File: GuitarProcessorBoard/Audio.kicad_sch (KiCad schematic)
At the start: 44 parts, among them U201 TLV320AIC3204, U202 TL074

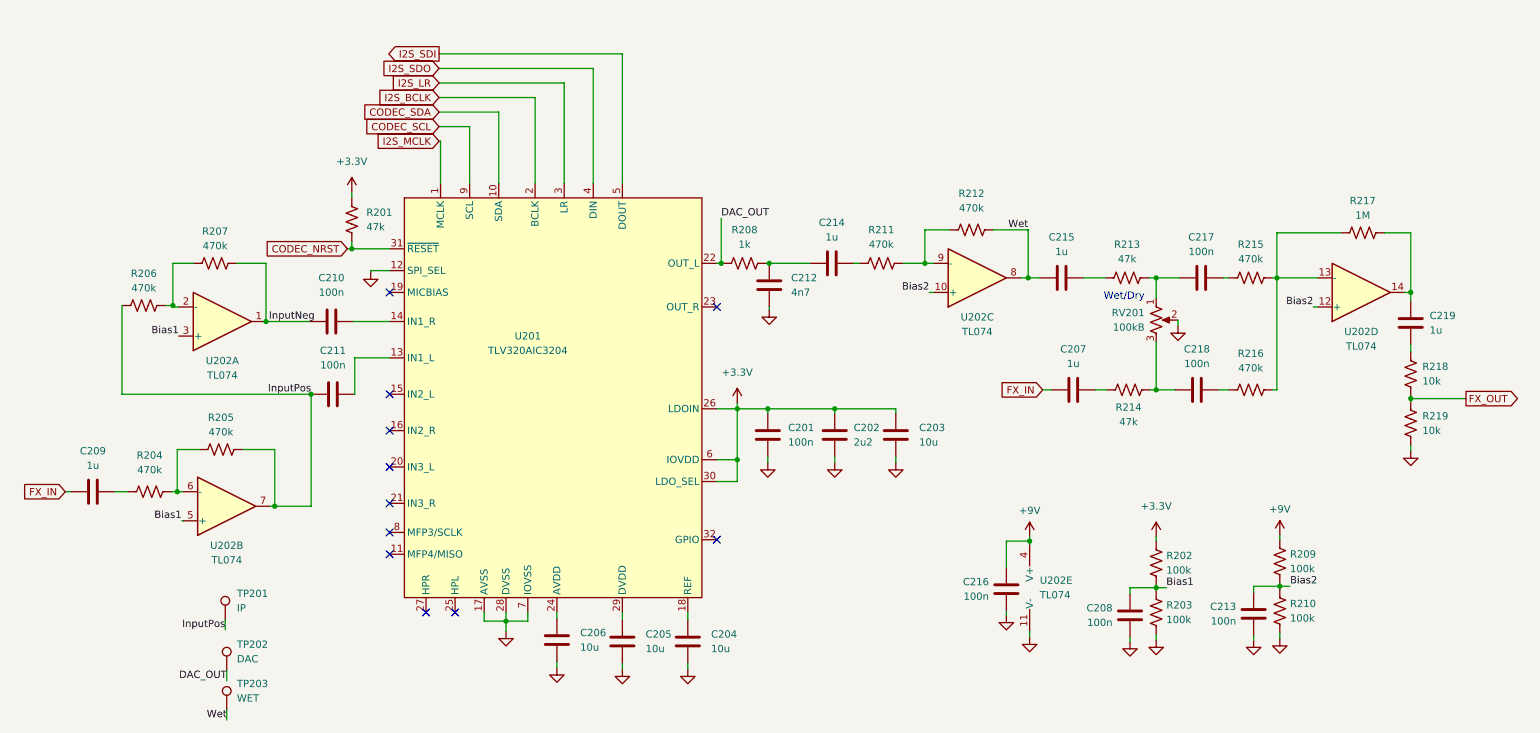
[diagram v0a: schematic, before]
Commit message: starting layout
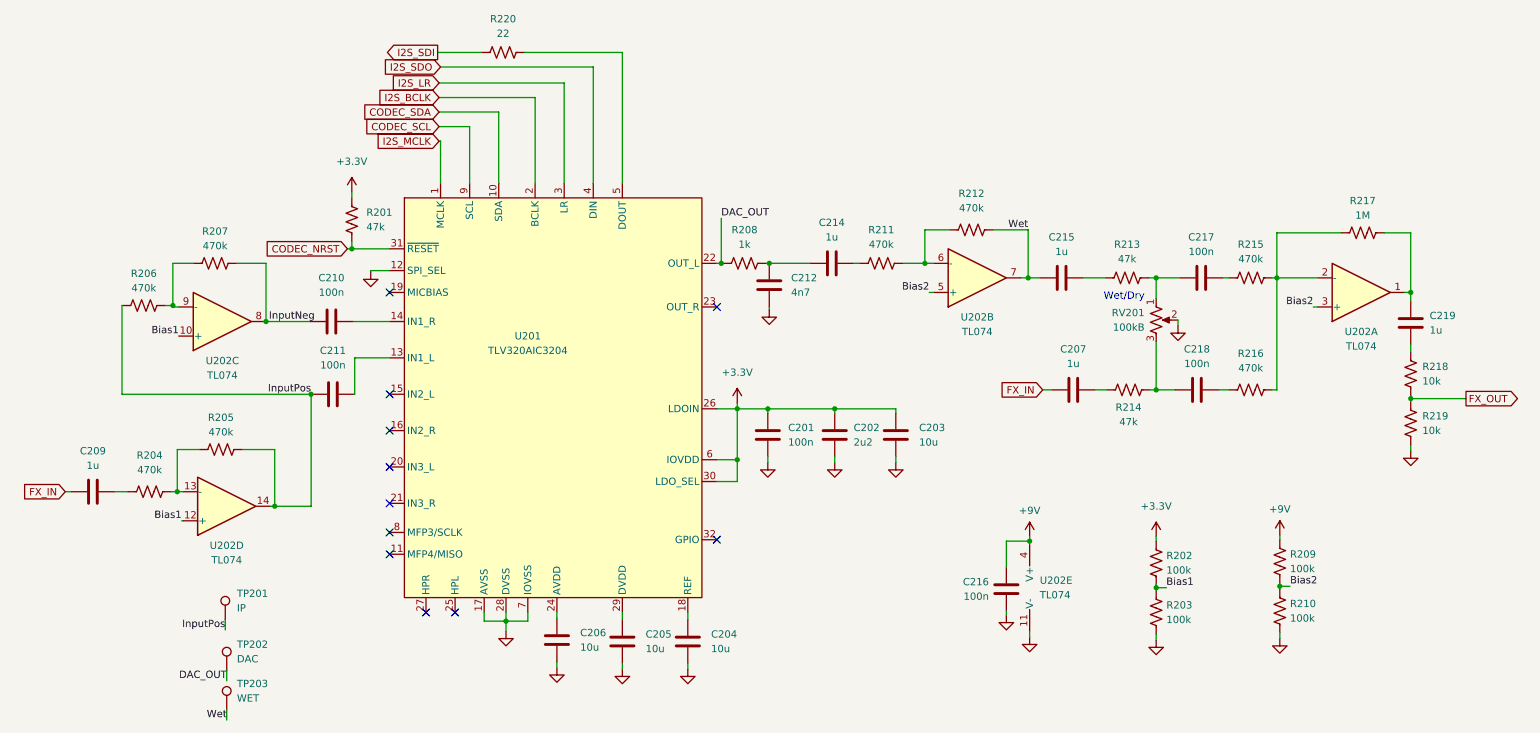
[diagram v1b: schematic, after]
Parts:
- removed C208, C213: 100n, Capacitor_SMD:C_0805_2012Metric, symbol Device:C
- added R220: 22, Resistor_SMD:R_0805_2012Metric, symbol Device:R_US
- RV201: footprint Potentiometer_THT:Potentiometer_Alpha_RV16AF_42_Single_Long -> Potentiometer_THT:Potentiometer_Alpha_RD901F-40-00D_Single_Vertical_CircularHoles
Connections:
- net Bias1: now also U202.10 (+), U202.12 (+); no longer U202.3 (+), U202.5 (+)
- net Bias2: now also U202.3 (+), U202.5 (+); no longer U202.10 (+), U202.12 (+)
- net I2S_SDI: now also R220.1; no longer U201.5 (DOUT)
- net InputNeg: now also U202.8; no longer U202.1
- net InputPos: now also U202.14; no longer U202.7
- net Wet: now also U202.7; no longer U202.8
- net at R206.2, R207.1: now also U202.9 (-); no longer U202.2 (-)
- net at R204.2, R205.1: now also U202.13 (-); no longer U202.6 (-)
- net at R211.2, R212.1: now also U202.6 (-); no longer U202.9 (-)
- net at R215.2, R216.2, R217.1: now also U202.2 (-); no longer U202.13 (-)
- net at C219.1, R217.2: now also U202.1; no longer U202.14
- new net: R220.2, U201.5 (DOUT)
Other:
- moved on the sheet: U202A, U202B, U202C, U202D
